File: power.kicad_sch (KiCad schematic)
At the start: 15 parts, among them U301 3.3, U302 TPS7B8733QKVURQ1

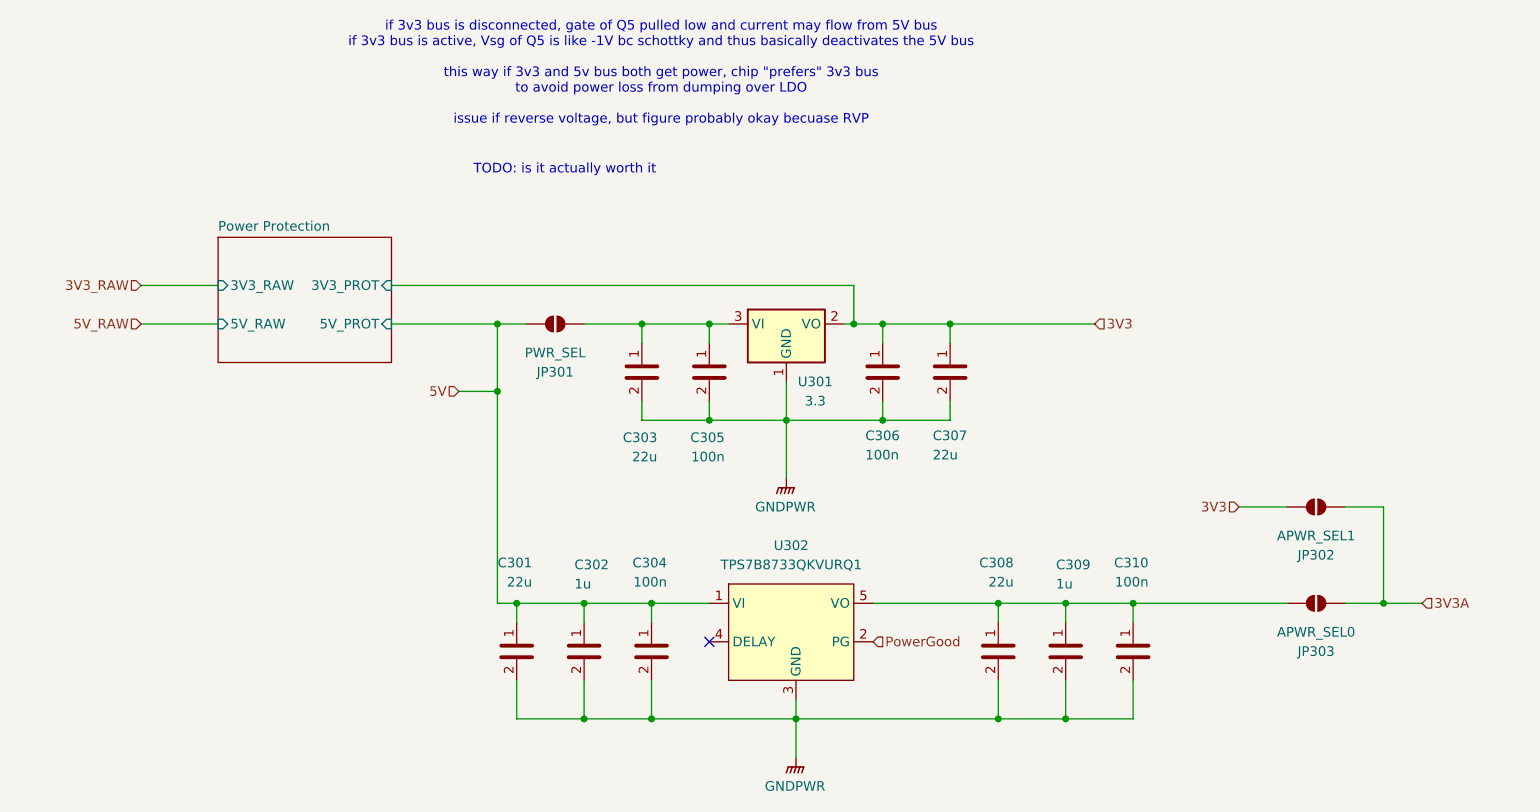
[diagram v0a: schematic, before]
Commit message: fixed like a bunch of things, power and new xcvr and lights and other goodies, also started layout
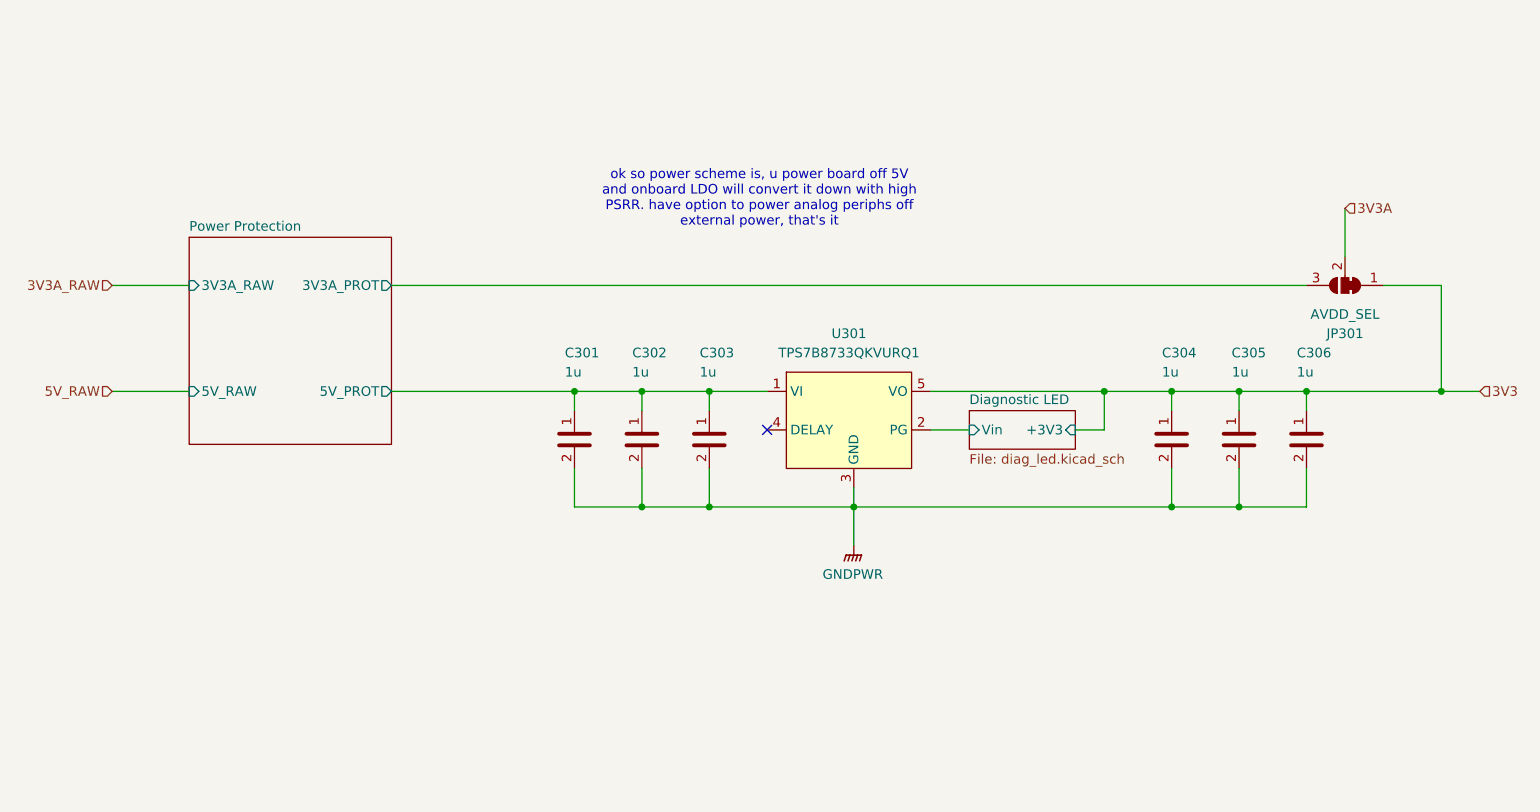
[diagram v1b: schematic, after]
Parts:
- removed C301, C303, C307, C308: 22u, Capacitor_SMD:C_0805_2012Metric_Pad1.18x1.45mm_HandSolder, symbol bfr_capacitors:CL21A226MAQNNNE
- removed C304, C305, C306, C310: 100n, Capacitor_SMD:C_0603_1608Metric_Pad1.08x0.95mm_HandSolder, symbol bfr_capacitors:06035C104KAT2A
- removed JP301: PWR_SEL, symbol Jumper:SolderJumper_2_Open
- removed JP302: APWR_SEL1, symbol Jumper:SolderJumper_2_Open
- removed JP303: APWR_SEL0, symbol Jumper:SolderJumper_2_Open
- removed U301: 3.3, Package_TO_SOT_SMD:SOT-223-3_TabPin2, symbol bfr_power_ics:AMS1117-3.3
- added C301, C303, C304, C306: 1u, Capacitor_SMD:C_0402_1005Metric_Pad0.74x0.62mm_HandSolder, symbol bfr_capacitors:CL05A105KA5NQNC
- added JP301: AVDD_SEL, Jumper:SolderJumper-3_P1.3mm_Bridged2Bar12_Pad1.0x1.5mm_NumberLabels, symbol Jumper:SolderJumper_3_Bridged12
- renumbered C309 to C305, U302 to U301
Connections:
- net 3V3: now also C305.1, U301.5 (VO), C304.1, C306.1, JP301.1 (A)
- net 3V3A: now also JP301.2 (C)
- net GNDPWR: now also C301.2, C303.2, C304.2, C306.2
- net 5V renamed Power Protection/5V_PROT
- net Power Protection/5V_PROT: now also C301.1, C303.1
- net PowerGood renamed Diagnostic LED/Vin
- new net Power Protection/3V3A_PROT: JP301.3 (B)
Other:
- added sheet Diagnostic LED (diag_led.kicad_sch)
- sheet Power Protection ports: added 3V3A_PROT, 3V3A_RAW; removed 3V3_PROT, 3V3_RAW
- note added: "ok so power scheme is, u power board off 5V and onboard LDO will convert it down with high PSRR. have option to power analog periphs off external power, that's it"
- note removed: "TODO: is it actually worth it"
- note removed: "if 3v3 bus is disconnected, gate of Q5 pulled low and current may flow from 5V bus if 3v3 bus is active, Vsg of Q5 is like -1V bc schottky and thus basically deactivates the 5V bus this way if 3v3 and 5v bus both get power, chip "prefers" 3v3 bus to avoid power loss from dumping over LDO issue if reverse voltage, but figure probably okay becuase RVP"
- moved on the sheet: C302, C305, U301
